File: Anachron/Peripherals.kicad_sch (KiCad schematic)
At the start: 21 parts, among them SW2 Pad, U4 BMI270, U5 MAX98357A

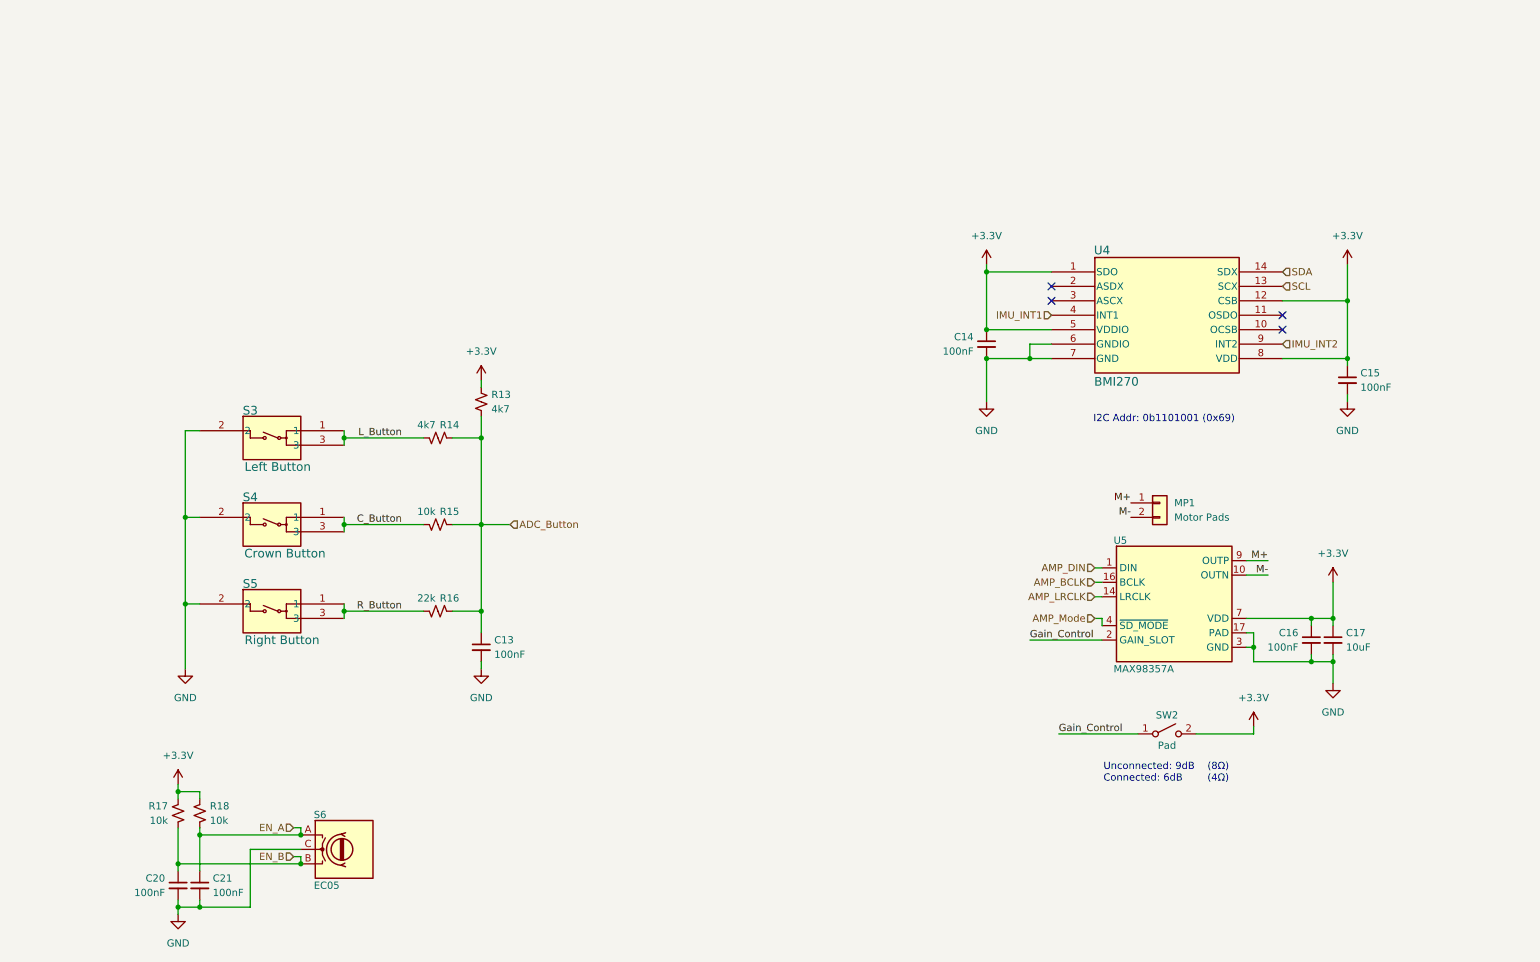
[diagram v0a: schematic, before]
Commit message: more changes!
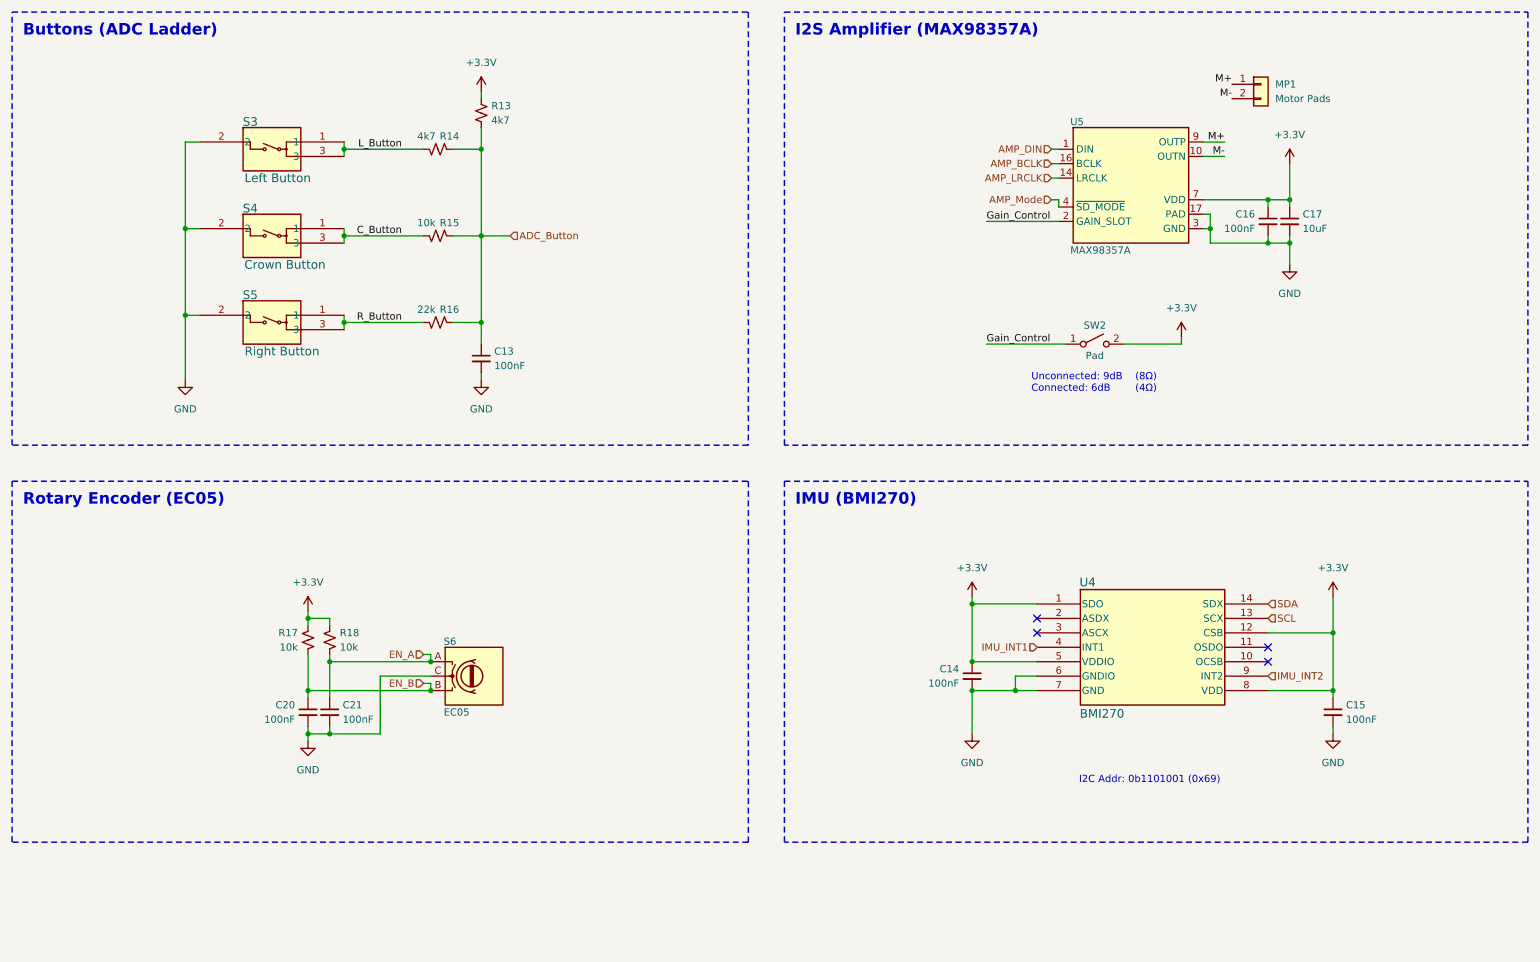
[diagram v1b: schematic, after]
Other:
- note added: "Buttons (ADC Ladder)"
- note added: "I2S Amplifier (MAX98357A)"
- note added: "IMU (BMI270)"
- note added: "Rotary Encoder (EC05)"
- moved on the sheet: C13, C14, C15, C16, C17, C20, C21, MP1, R13, R14, R15, R16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
